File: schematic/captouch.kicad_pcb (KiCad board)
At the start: 2 copper layers, 26 x 40 mm, 18 parts, among them P1 POWER, P2 PROGRAM, P3 LAMP, Q1 DMN3404L, U1 LD1117S33CTR, U2 MSP430G2553IPW20

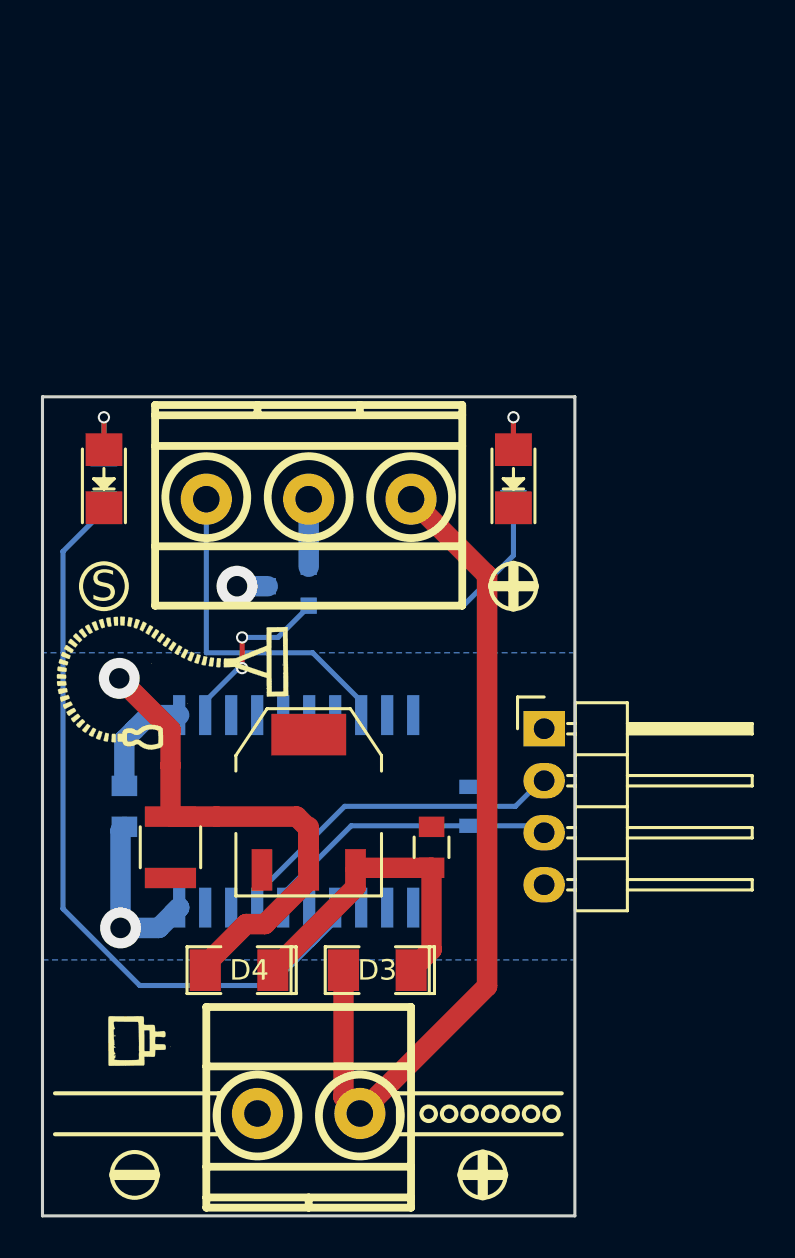
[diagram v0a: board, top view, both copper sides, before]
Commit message: More little adjustments + logo
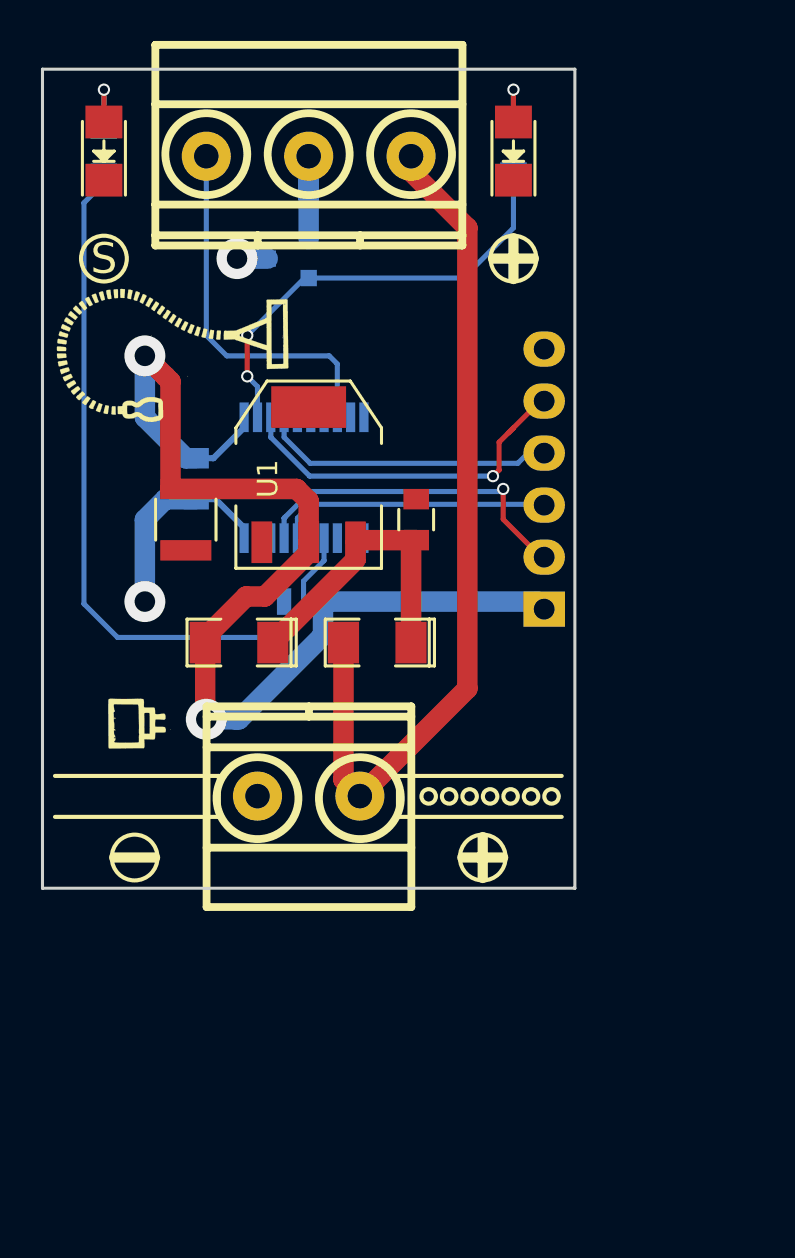
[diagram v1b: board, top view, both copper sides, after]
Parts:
- removed G***: LOGO, logo:lamp
- added ?: , logo:lamp, F.Cu at (58.5, 32.8)
- added ?: , logo:wpd, B.Cu at (56.0, 54.0)
- ?: renamed from G***; value LOGO -> (none)
- P1: footprint w_conn_mkds:mkds_1,5-2 -> conn:P_1,5-2
- P2: footprint Pin_Headers:Pin_Header_Angled_1x04 -> Pin_Headers:Pin_Header_Angled_1x06; moved to B.Cu
- P3: footprint w_conn_mkds:mkds_1,5-3 -> conn:P_1,5-3
- U2: footprint Housings_SOIC:SOIC-20_7.5x12.8mm_Pitch1.27mm -> Housings_SSOP:TSSOP-20_4.4x6.5mm_Pitch0.65mm
- moved P3 16.8 mm to (65.0, 23.2)
- moved C3 16.4 mm to (59.5, 39.0)
- moved U2 16.3 mm to (64.8, 39.0)
- moved C1 16.0 mm to (70.2, 41.0)
- moved C2 16.0 mm to (59.0, 41.0)
- moved R2 16.0 mm to (75.0, 22.9)
- moved D1 16.0 mm to (75.0, 23.0)
- moved D2 16.0 mm to (55.0, 23.0)
- moved D3 16.0 mm to (68.3, 47.0)
- moved D4 16.0 mm to (61.6, 47.0)
- moved Q1 16.0 mm to (64.0, 28.2)
- moved R3 16.0 mm to (55.0, 23.0)
- moved U1 16.0 mm to (65.0, 38.8)
- moved ? 15.5 mm to (56.5, 50.0)
- moved P1 15.5 mm to (65.0, 54.5)
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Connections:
- P2 pad 4: GNDREF -> RXD
- U2 pad 3: (no net) -> TXD
- U2 pad 4: (no net) -> RXD
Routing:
- net +3V3: track 31.7 -> 57.1 mm, vias 1 -> 2
- net TXD: track 0.00 -> 17.8 mm, vias 0 -> 1
- net RXD: track 0.00 -> 14.6 mm
- net Net-(P3-Pad3): track 16.0 -> 19.1 mm
- net Net-(P3-Pad2): track 3.30 -> 5.30 mm
- net /RST: track 14.9 -> 16.7 mm
- net Net-(D3-Pad2): track 41.4 -> 43.1 mm
- net GNDREF: track 10.2 -> 11.8 mm
- net Net-(C1-Pad1): track 14.9 -> 13.8 mm
- net Net-(R3-Pad2): track 38.7 -> 38.1 mm
- net TEST: track 17.0 -> 16.8 mm, vias 0 -> 1
- removed copper zone on B.Cu, net +3V3
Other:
- board text added: "201605"
- board text added: "3V3"
- board text added: "GND"
- board text added: "RST"
- board text added: "RX"
- board text added: "TST"
- board text added: "TX"
- board text removed: "WPD 201605"
